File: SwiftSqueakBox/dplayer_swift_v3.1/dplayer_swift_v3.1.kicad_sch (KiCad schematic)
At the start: 10 parts, among them SW1 Reset, U1 ATtiny85-20P, U2 dfplayer

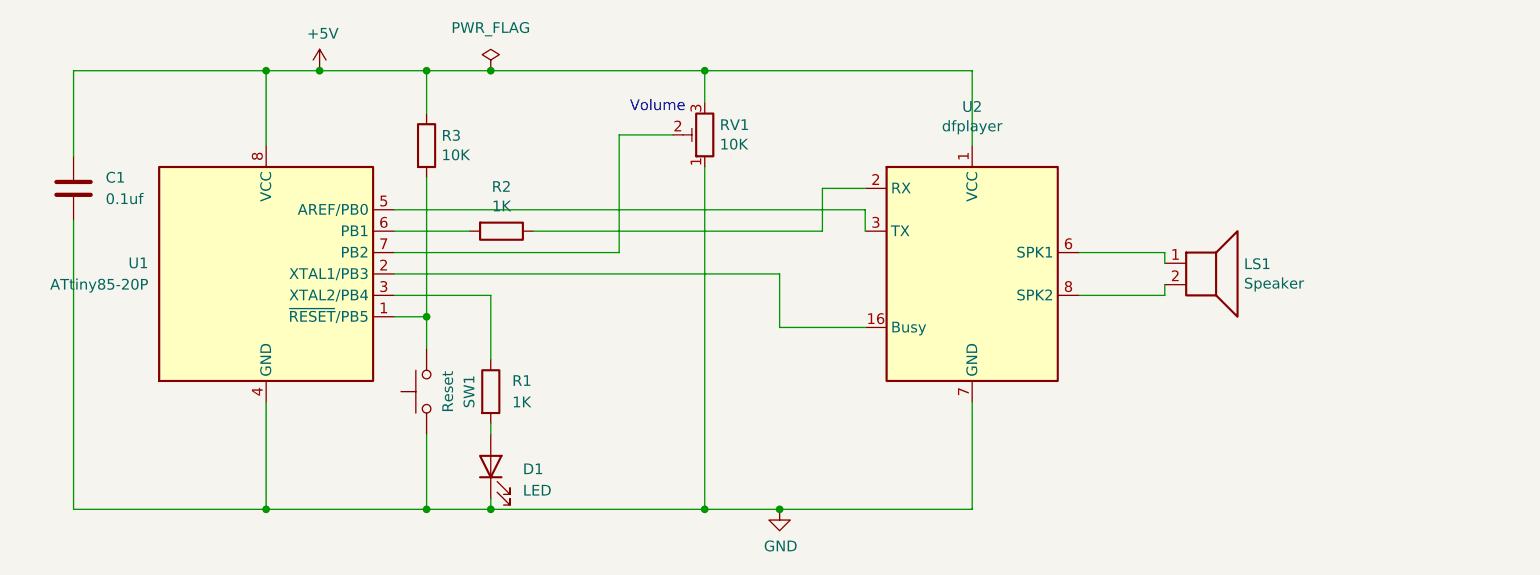
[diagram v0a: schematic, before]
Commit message: update pcb and schematic
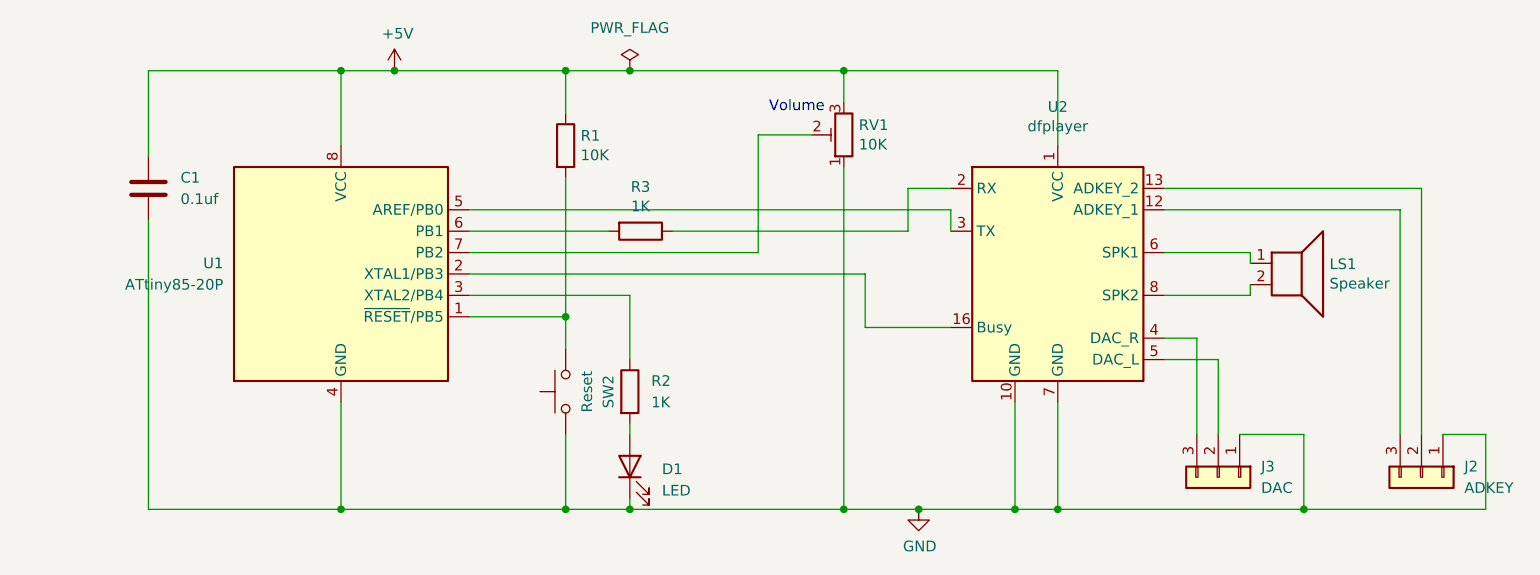
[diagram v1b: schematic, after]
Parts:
- added J2: ADKEY, Connector_PinHeader_2.00mm:PinHeader_1x03_P2.00mm_Vertical, symbol Connector_Generic:Conn_01x03
- added J3: DAC, Connector_PinHeader_2.00mm:PinHeader_1x03_P2.00mm_Vertical, symbol Connector_Generic:Conn_01x03
- renumbered R3 to R1, R1 to R2, R2 to R3, SW1 to SW2
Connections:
- net GND: now also U2.10 (GND), J2.1 (Pin_1), J3.1 (Pin_1)
- new net: J2.3 (Pin_3), U2.12 (ADKEY_1)
- new net: J2.2 (Pin_2), U2.13 (ADKEY_2)
- new net: J3.3 (Pin_3), U2.4 (DAC_R)
- new net: J3.2 (Pin_2), U2.5 (DAC_L)
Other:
- title: Gierzwaluw lokker v3 -> Swift Squeak Box v3.1
- moved on the sheet: C1, D1, LS1, R1, R2, R3, RV1, SW2, U1
